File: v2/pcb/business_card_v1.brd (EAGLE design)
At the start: 89 x 51 mm, 70 parts, among them SW1 SPST_TACT-KMR2

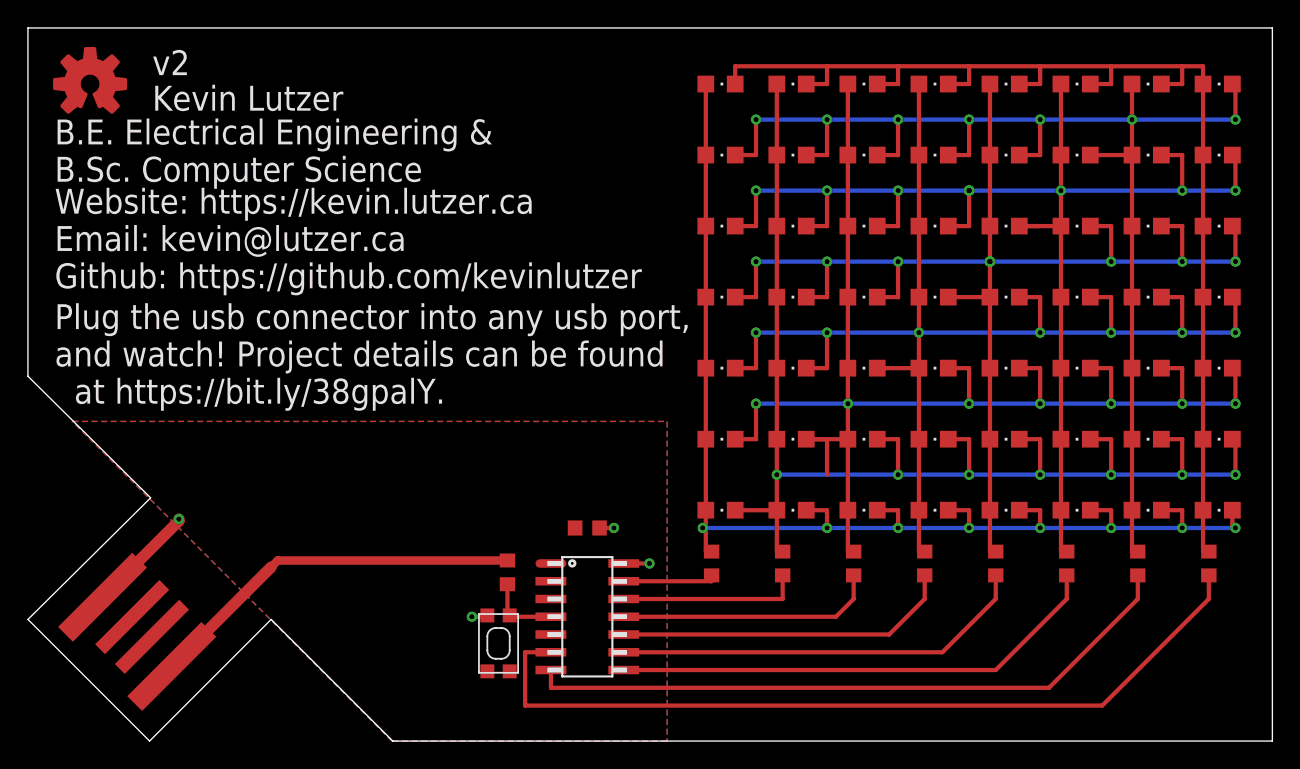
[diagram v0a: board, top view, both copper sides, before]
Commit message: business card
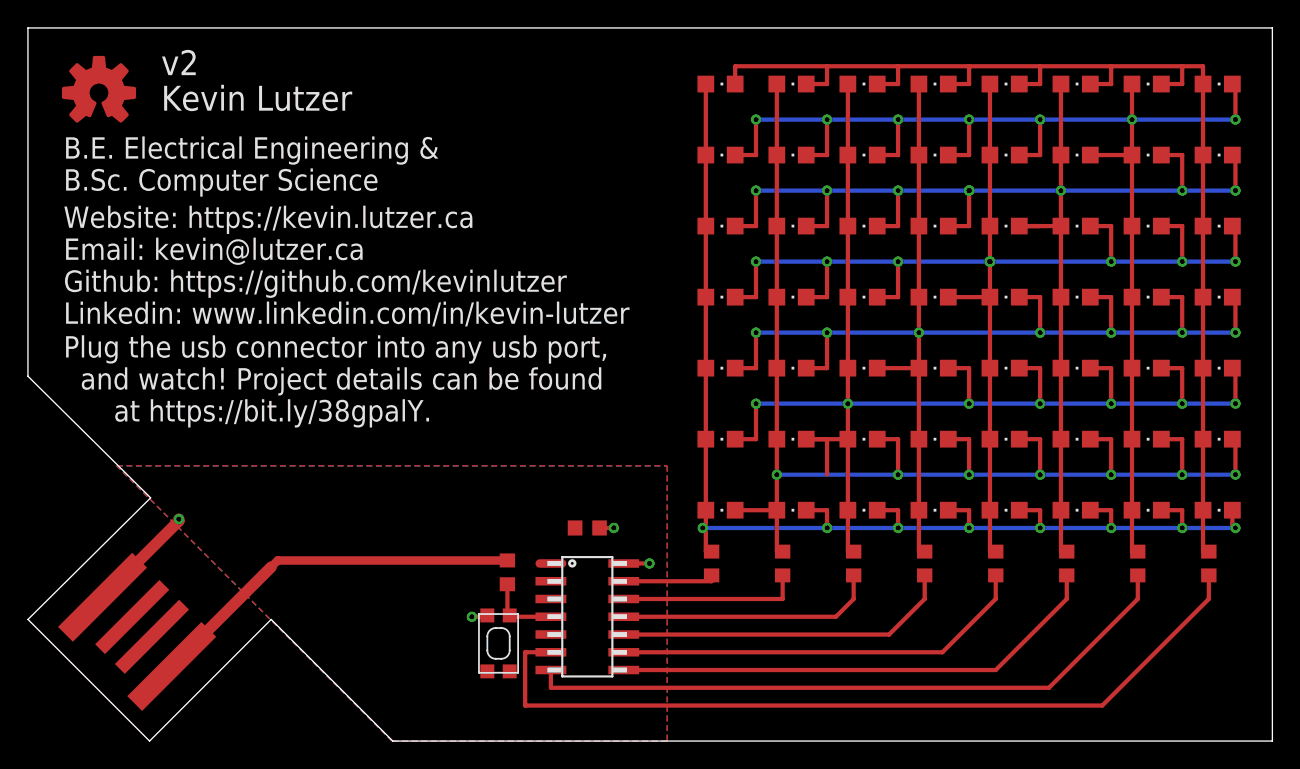
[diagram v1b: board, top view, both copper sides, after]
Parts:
- moved U$1 0.90 mm to (5.08, 46.4)
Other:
- board text added: "Website: https://kevin.lutzer.ca Email: kevin@lutzer.ca Github: https://github.com/kevinlutzer Linkedin: www.linkedin.com/in/kevin-lutzer"
- board text removed: "Website: https://kevin.lutzer.ca Email: kevin@lutzer.ca Github: https://github.com/kevinlutzer"
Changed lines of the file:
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@@
 <dimension x1="0" y1="51.79" x2="89" y2="51.79" x3="44.5" y3="56.79" textsize="1" layer="1"/>
 <dimension x1="89" y1="51.79" x2="89" y2="0.79" x3="94" y3="26.29" textsize="1" layer="1"/>
-<text x="8.89" y="47.625" size="1.778" layer="121">v2</text>
-<text x="8.89" y="45.085" size="1.778" layer="121">Kevin Lutzer</text>
-<text x="1.905" y="40.005" size="1.778" layer="121">B.E. Electrical Engineering &amp;
+<text x="9.525" y="47.625" size="1.778" layer="121">v2</text>
+<text x="9.525" y="45.085" size="1.778" layer="121">Kevin Lutzer</text>
+<text x="2.54" y="39.37" size="1.524" layer="121">B.E. Electrical Engineering &amp;
 B.Sc. Computer Science</text>
-<text x="1.905" y="32.385" size="1.778" layer="121">Website: https://kevin.lutzer.ca
+<text x="2.54" y="29.845" size="1.524" layer="121">Website: https://kevin.lutzer.ca
 Email: kevin@lutzer.ca
-Github: https://github.com/kevinlutzer</text>
-<text x="1.905" y="24.13" size="1.778" layer="121">Plug the usb connector into any usb port,
-and watch! Project details can be found
-  at https://bit.ly/38gpalY.</text>
+Github: https://github.com/kevinlutzer
+Linkedin: www.linkedin.com/in/kevin-lutzer</text>
+<text x="2.54" y="22.86" size="1.524" layer="121">Plug the usb connector into any usb port,
+  and watch! Project details can be found
+      at https://bit.ly/38gpalY.</text>
 </plain>
 <attributes>
@@
 <attribute name="VALUE" x="38.6715" y="12.3825" size="1.27" layer="27" ratio="10" rot="R270"/>
 </element>
-<element name="U$1" library="adafruit" library_urn="urn:adsk.eagle:library:420" package="OSHWLOGO_TOP_0.2" package3d_urn="urn:adsk.eagle:package:6240813/1" value="" x="4.445" y="46.99" smashed="yes"/>
+<element name="U$1" library="adafruit" library_urn="urn:adsk.eagle:library:420" package="OSHWLOGO_TOP_0.2" package3d_urn="urn:adsk.eagle:package:6240813/1" value="" x="5.08" y="46.355" smashed="yes"/>
 </elements>
 <signals>
@@
 <contactref element="IC1" pad="14"/>
 <polygon width="0.6096" layer="16">
-<vertex x="3.175" y="22.86"/>
-<vertex x="45.72" y="22.86"/>
+<vertex x="6.35" y="19.685"/>
+<vertex x="45.72" y="19.685"/>
 <vertex x="45.72" y="0"/>
 <vertex x="26.035" y="0"/>
@@
 <wire x1="17.864746875" y1="12.915" x2="34.29" y2="12.915" width="0.6096" layer="1"/>
 <polygon width="0.6096" layer="1">
-<vertex x="3.175" y="22.86"/>
-<vertex x="45.72" y="22.86"/>
+<vertex x="6.35" y="19.685"/>
+<vertex x="45.72" y="19.685"/>
 <vertex x="45.72" y="0"/>
 <vertex x="26.035" y="0"/>
